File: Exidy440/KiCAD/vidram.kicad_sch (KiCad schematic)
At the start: 35 parts, among them U10J 74LS74, U10K 74LS161, U10L 74LS32, U11J 74LS02, U11K 74LS161, U13K 74LS173, U13L 74LS157, U14K 74LS173, U14L MN2114, U15K 74LS374, U15L MN2114, U16K 74LS244, U16L MN2114, U17K 74LS245, U17L 74LS374, U18A 74LS189, U18K 74LS273, U18L 74LS273, U19A 74LS189, U20A 74LS189, U21A 74LS189, U22A 74LS169, U22F 74LS30, U22H 74LS283, U23C 74LS04, U23D 74LS08, U23F 74LS189, U23H 74LS283, U2L 74LS04, U5J 74LS04, U9K 74LS161

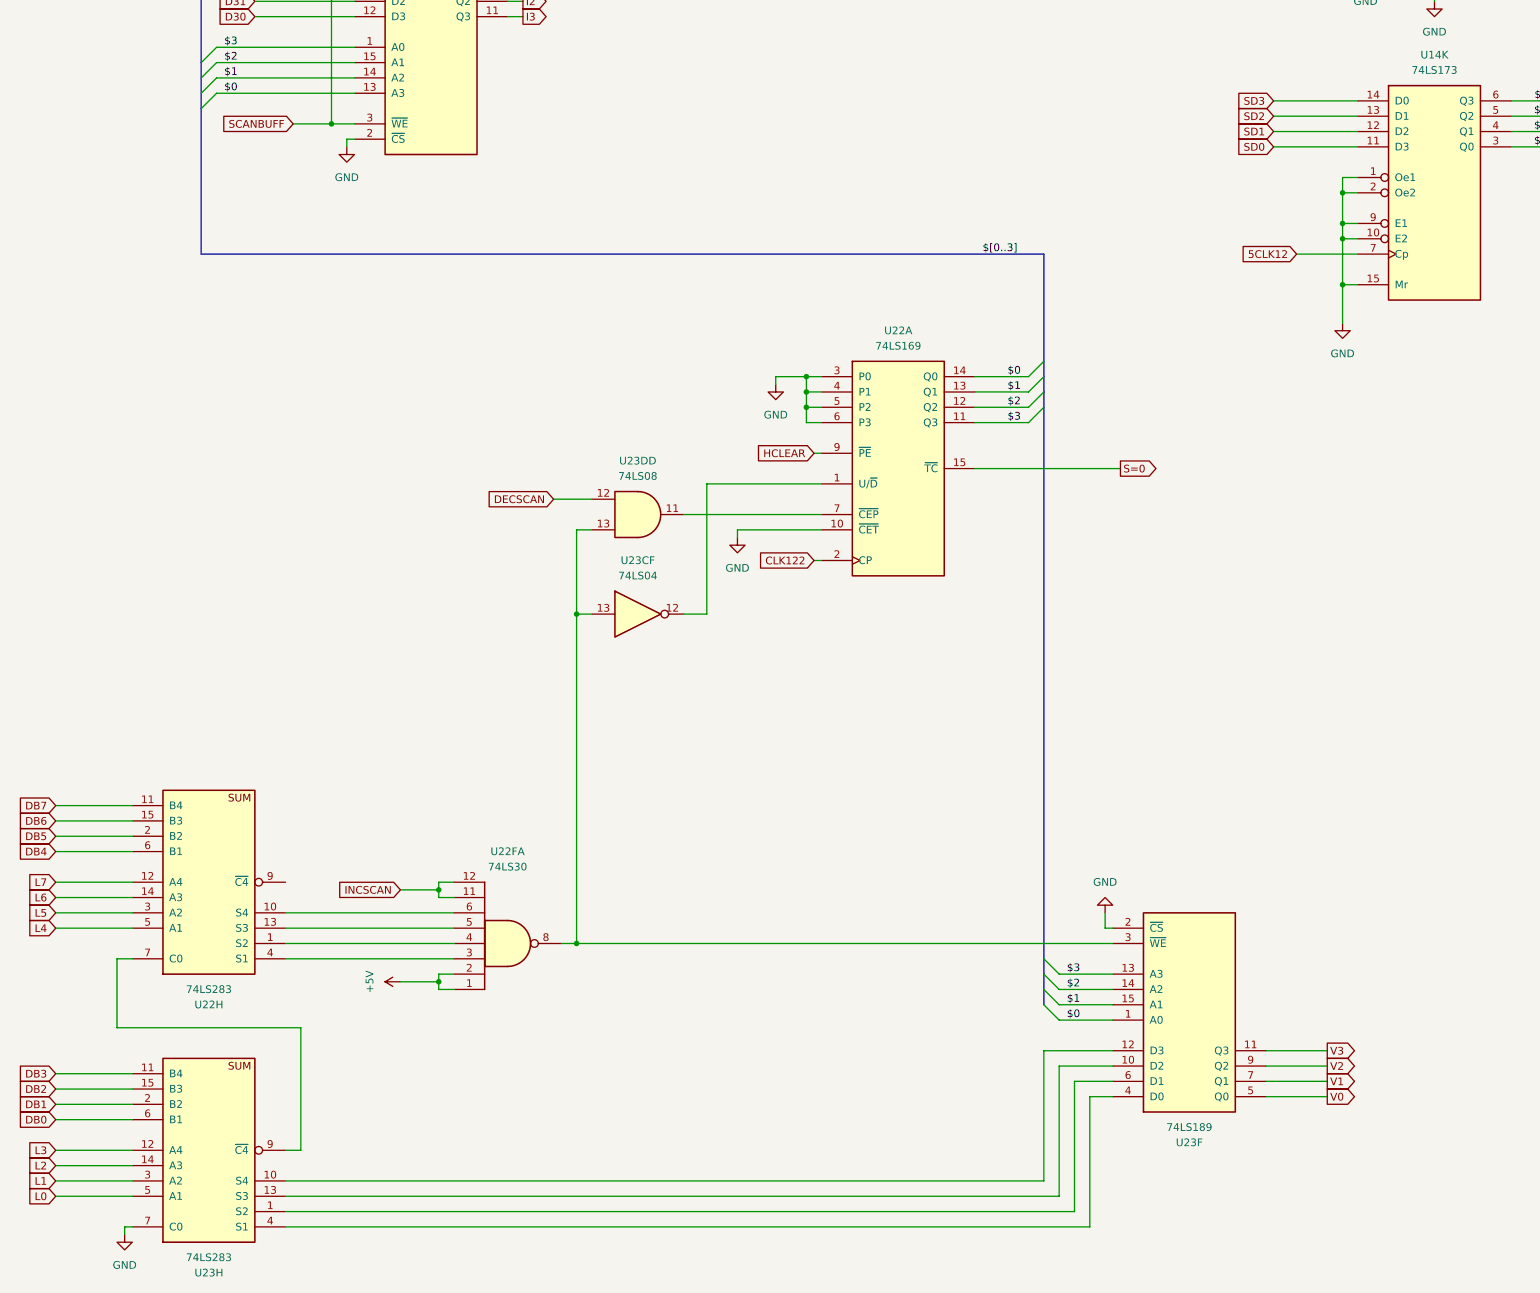
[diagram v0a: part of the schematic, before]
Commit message: Minor modifications to IO board
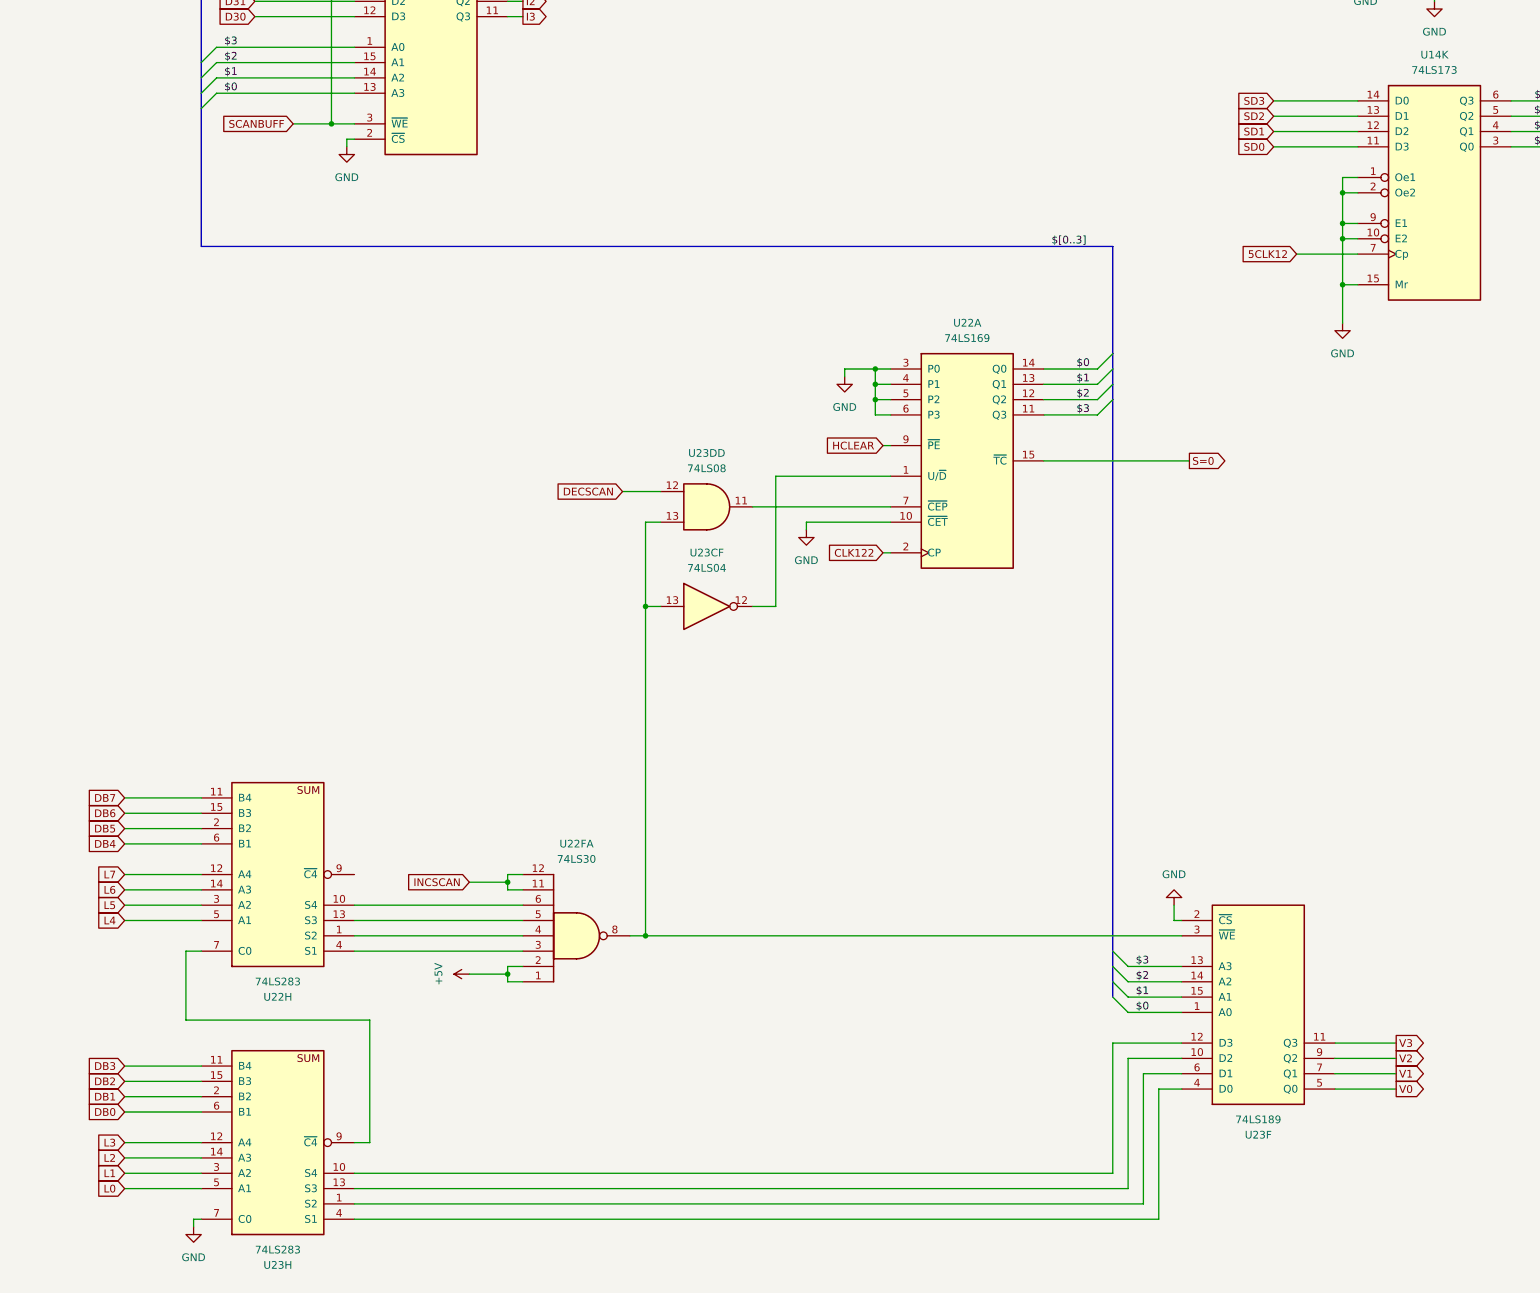
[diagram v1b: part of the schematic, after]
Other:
- moved on the sheet: U22A, U22FA, U22H, U23CF, U23DD, U23F, U23H
